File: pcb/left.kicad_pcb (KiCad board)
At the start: 2 copper layers, 135 x 95.7 mm, 55 parts, among them SW1 SW_PUSH, SW10 SW_PUSH, SW11 SW_PUSH, SW12 SW_PUSH, SW13 SW_PUSH, SW14 SW_PUSH, SW15 SW_PUSH, SW16 SW_PUSH, SW17 SW_PUSH, SW18 SW_PUSH, SW19 SW_PUSH, SW2 SW_PUSH, SW20 SW_PUSH, SW3 SW_PUSH, SW4 SW_PUSH, SW5 SW_PUSH, SW6 SW_PUSH, SW7 SW_PUSH, SW8 SW_PUSH, SW9 SW_PUSH, U1 xiao-ble

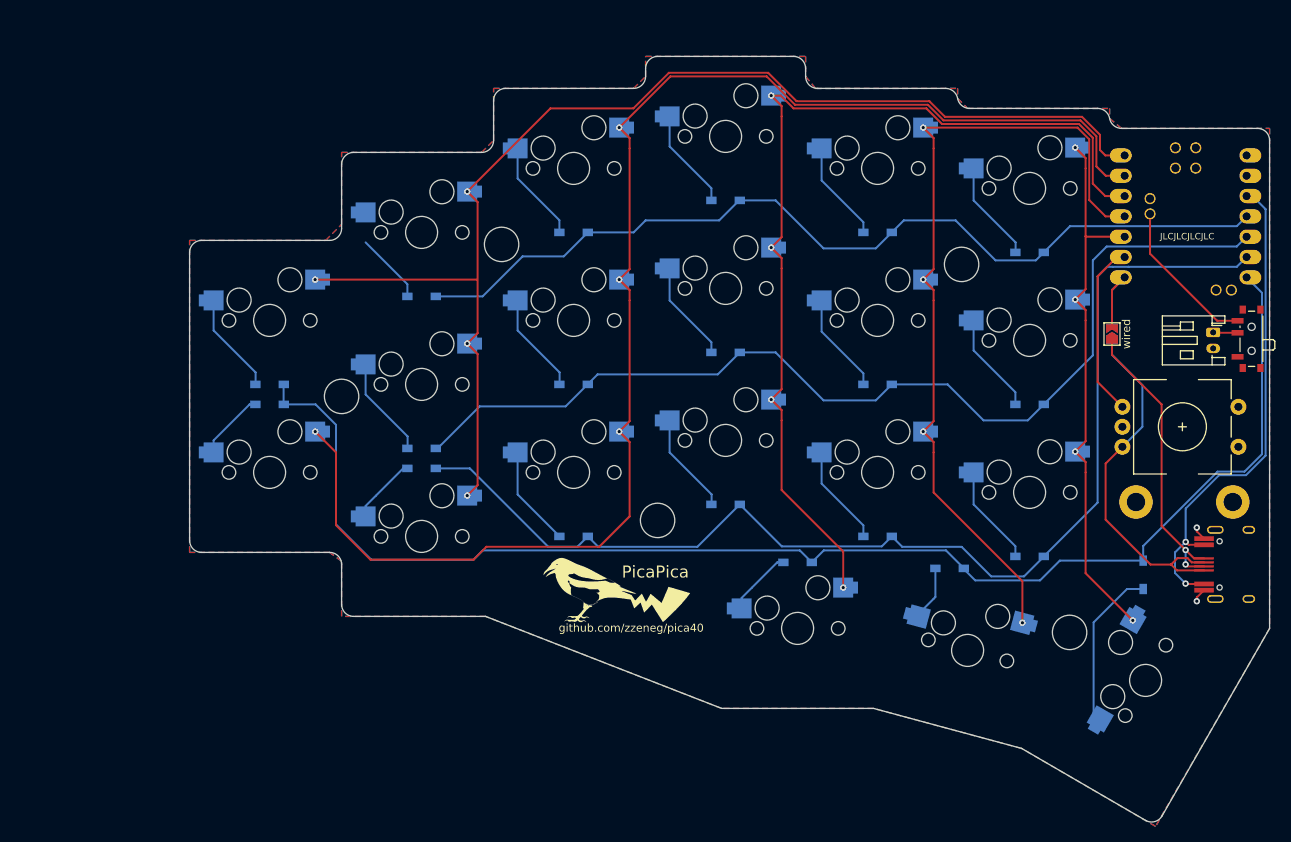
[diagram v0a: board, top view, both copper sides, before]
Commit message: v2
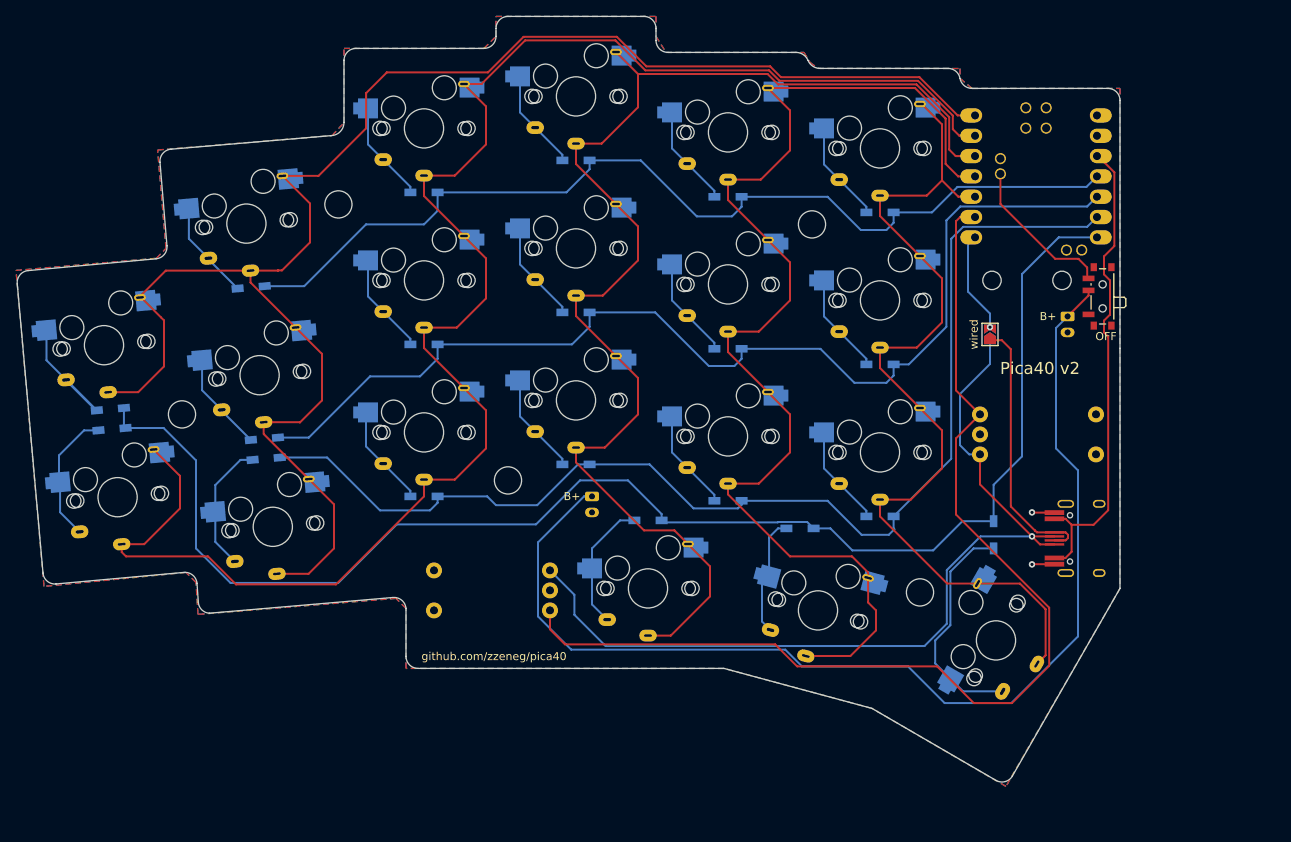
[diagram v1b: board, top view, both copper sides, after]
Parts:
- removed wired, wireless: SolderJumper_2_Open, Jumper:SolderJumper-2_P1.3mm_Open_TrianglePad1.0x1.5mm
- added BATTCONN2: Conn_01x02_Female, pica:JST_PH_S2B-PH-K_1x02_P2.00mm, F.Cu at (118.8, 105.5)
- added JP1: SolderJumper_2_Open, Jumper:SolderJumper-2_P1.3mm_Open_TrianglePad1.0x1.5mm, B.Cu at (168.6, 85.2)
- added JP2: SolderJumper_2_Open, Jumper:SolderJumper-2_P1.3mm_Open_TrianglePad1.0x1.5mm, F.Cu at (168.6, 85.2)
- added RE2: RotaryEncoder_Switch, pica:RotaryEncoder_EC11, F.Cu at (106.0, 117.2)
- BATTCONN1: footprint Connector_JST:JST_PH_S2B-PH-K_1x02_P2.00mm_Horizontal -> pica:JST_PH_S2B-PH-K_1x02_P2.00mm
- G***: moved to B.Cu
- H1, H2, H3, H4, H5: footprint kbd:M2_HOLE_v2 -> pica:spacer_m2_3.4
- H6, H7: footprint kbd:M2_Hole_TH -> kbd:thread_m2
- SW1, SW10, SW11, SW12, SW13, SW14, SW15, SW16, SW17, SW18, SW19, SW2, SW3, SW4, SW5, SW6, SW7, SW8, SW9: footprint pica:CherryMX_Hotswap -> pica:CherryMX_Hotswap_ChocV2
- SW20: footprint pica:CherryMX_Hotswap_1.5 -> pica:CherryMX_Hotswap_ChocV2_1.5
- U1: footprint kleeb-mcu:xiao-ble-tht -> pica:xiao-ble-tht
- moved H7 35.0 mm to (177.6, 78.5)
- moved H6 33.0 mm to (168.8, 78.5)
- moved SW1 21.9 mm to (75.6, 71.4), turned to 5 degrees
- moved D1 21.3 mm to (76.2, 79.4), turned to -175 degrees
- moved H1 21.0 mm to (87.1, 69.0)
- moved SW16 20.9 mm to (57.8, 86.6), turned to 5 degrees
- moved SW6 20.3 mm to (77.2, 90.3), turned to 5 degrees
- moved D16 20.1 mm to (58.6, 94.6), turned to -175 degrees
- moved H3 20.1 mm to (67.5, 95.2), turned to 5 degrees
- moved D17 19.9 mm to (58.8, 97.1), turned to -175 degrees
- moved D6 19.7 mm to (77.9, 98.3), turned to -175 degrees
- moved D11 19.5 mm to (78.1, 100.8), turned to -175 degrees
- moved D18 19.4 mm to (125.8, 108.5)
- moved BATTSW1 19.4 mm to (182.3, 80.5)
- moved D12 19.4 mm to (97.8, 105.5)
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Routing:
- net BATT: track 3.07 -> 139.9 mm
- net ENCA: track 22.0 -> 136.0 mm
- net ENCB: track 45.6 -> 111.9 mm, vias 0 -> 1
- net col0: track 154.3 -> 208.8 mm, vias 4 -> 0
- net col4: track 69.1 -> 115.0 mm, vias 4 -> 0
- net col3: track 103.4 -> 148.0 mm, vias 4 -> 0
- net col2: track 120.1 -> 158.9 mm, vias 4 -> 0
- net col1: track 178.0 -> 210.6 mm, vias 4 -> 0
- net Net-(D20-Pad2): track 20.3 -> 28.7 mm
- net Net-(D17-Pad2): track 8.61 -> 16.9 mm
- net Net-(D19-Pad2): track 6.89 -> 15.0 mm
- net Net-(D18-Pad2): track 8.37 -> 16.4 mm
- net Net-(D11-Pad2): track 8.47 -> 16.5 mm
- net row0: track 114.5 -> 122.4 mm
- net row1: track 128.0 -> 135.4 mm
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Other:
- board size 135 x 95.7 mm -> 137.8 x 95.7 mm
- board text added: "B+"
- board text added: "OFF"
- board text added: "Pica40 v2"
- board text added: "wired"
- board text added: "wireless"
- board text removed: "JLCJLCJLCJLC"
- board text removed: "PicaPica"
